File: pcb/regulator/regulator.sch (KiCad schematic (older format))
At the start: 16 parts, among them J1 Conn_01x04, J2 Conn_01x03, SW1 SW_Push, U1 STM32G071CBT6, Y1 32kHz, Y2 8MHz

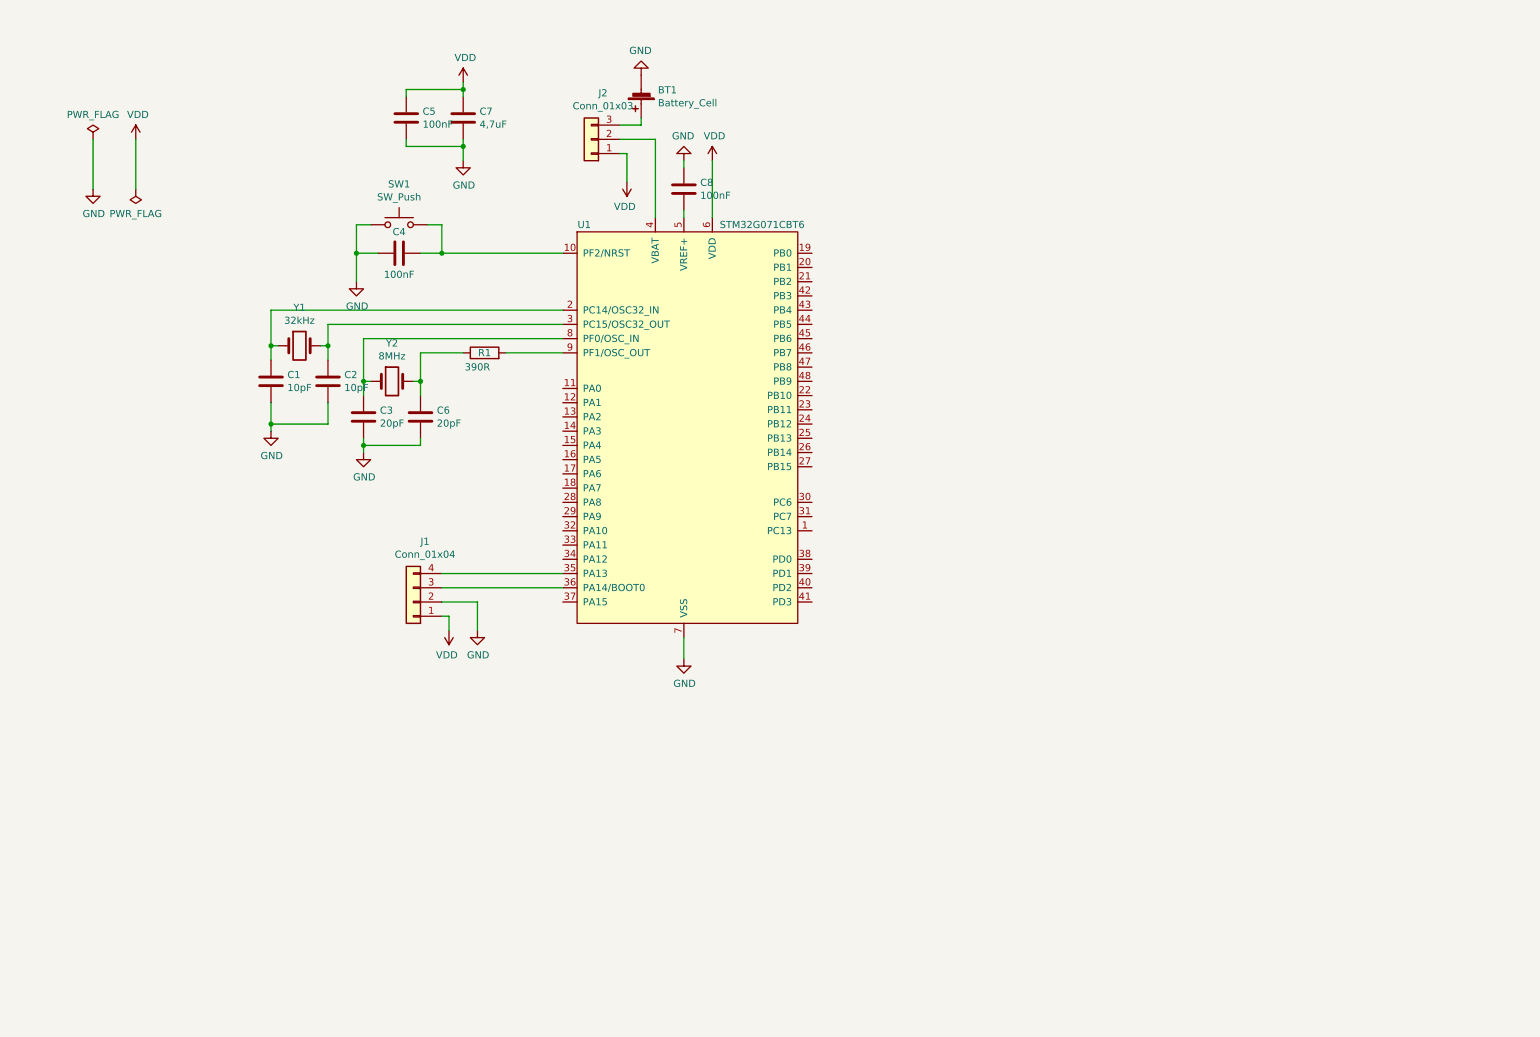
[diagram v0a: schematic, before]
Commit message: Device Schematic v1
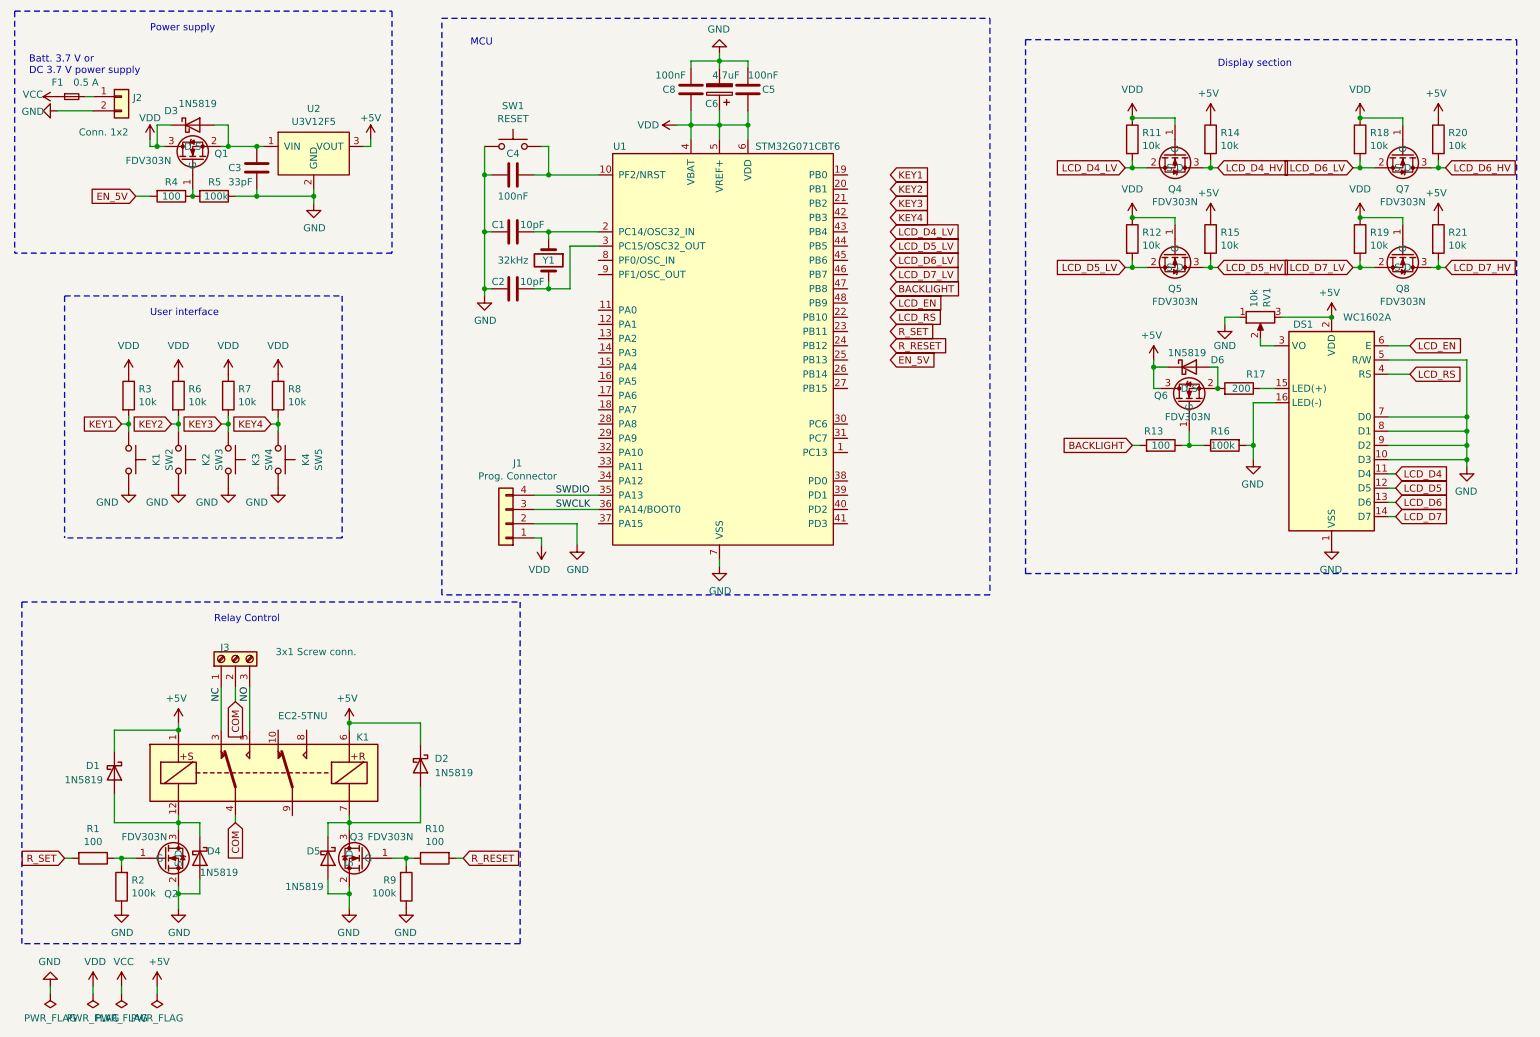
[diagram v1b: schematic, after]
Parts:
- removed BT1: Battery_Cell, symbol Device:Battery_Cell
- removed C6: 20pF, symbol Device:C
- removed C7: 4,7uF, symbol Device:C
- removed J2: Conn_01x03, symbol Connector_Generic:Conn_01x03
- removed Y2: 8MHz, symbol Device:Crystal
- added C6: 4.7uF, symbol Device:CP
- added D1, D2, D3, D4, D5, D6: 1N5819, Diode_THT:D_DO-41_SOD81_P10.16mm_Horizontal, symbol Diode:1N5819
- added DS1: WC1602A, Display:WC1602A, symbol Display_Character:WC1602A
- added F1: 0.5 A, symbol Device:Fuse_Small
- added J2: Conn. 1x2, symbol Connector_Generic:Conn_01x02
- added J3: 3x1 Screw conn., symbol Connector:Screw_Terminal_01x03
- added K1: EC2-5TNU, Relay_THT:Relay_DPDT_Kemet_EC2_DoubleCoil, symbol Relay:EC2-5TNU
- added Q1, Q2, Q3, Q4, Q5, Q6, Q7, Q8: FDV303N, Package_TO_SOT_SMD:SOT-23, symbol things:FDV303N
- added R10, R13, R4: 100, symbol Device:R
- added R11, R12, R14, R15, R18, R19, R20, R21, R3, R6, R7, R8: 10k, symbol Device:R
- added R16, R2, R5, R9: 100k, symbol Device:R
- added R17: 200, symbol Device:R
- added RV1: 10k, symbol Device:R_POT
- added SW2: K1, symbol Switch:SW_Push
- added SW3: K2, symbol Switch:SW_Push
- added SW4: K3, symbol Switch:SW_Push
- added SW5: K4, symbol Switch:SW_Push
- added U2: U3V12F5, Connector_PinHeader_2.54mm:PinHeader_1x03_P2.54mm_Vertical_SMD_Pin1Left, symbol things:U3V12F5
- C3: value 20pF -> 33pF
- J1: value Conn_01x04 -> Prog. Connector
- R1: value 390R -> 100
- SW1: value SW_Push -> RESET
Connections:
- net GND: now also C5.1, C6.2, D4.2 (A), D5.2 (A), DS1.1 (VSS), DS1.10 (D3), DS1.16 (LED(-)), DS1.5 (R/W), DS1.7 (D0), DS1.8 (D1), DS1.9 (D2), J2.2 (Pin_2), Q2.2 (S), Q3.2 (S), R16.2, R2.1, R5.1, R9.1, RV1.1, SW2.2, SW3.2, SW4.2, SW5.2, U2.2 (GND); no longer C5.2
- net VDD: now also C5.2, C8.2, U1.4 (VBAT), U1.5 (VREF+), C6.1, D3.1 (K), Q1.3 (D), Q4.1 (G), Q5.1 (G), Q7.1 (G), Q8.1 (G), R11.1, R12.1, R18.1, R19.1, R3.1, R6.1, R7.1, R8.1; no longer C5.1
- net SWDIO: now reaches J1.4 (Pin_4), U1.35 (PA13)
- net SWCLK: now reaches J1.3 (Pin_3), U1.36 (PA14/BOOT0)
- net at U1.8 (PF0/OSC_IN): no longer C3.1
- net at U1.9 (PF1/OSC_OUT): no longer R1.2
- net at R1.1: now also Q2.1 (G), R2.2
- new net: Q1.1 (G), R4.1, R5.2
- new net: C3.1, D3.2 (A), Q1.2 (S), U2.1 (VIN)
- new net: D1.2 (A), D4.1 (K), K1.12, Q2.3 (D)
- new net: Q3.1 (G), R10.1, R9.2
- new net: D2.2 (A), D5.1 (K), K1.7, Q3.3 (D)
- new net: Q6.1 (G), R13.1, R16.1
- new net: DS1.15 (LED(+)), R17.1
- new net: D6.2 (A), Q6.2 (S), R17.2
- new net: DS1.3 (VO), RV1.2
- new net: F1.2, J2.1 (Pin_1)
- new net +5V: D1.1 (K), D2.1 (K), D6.1 (K), DS1.2 (VDD), K1.1, K1.6, Q6.3 (D), R14.1, R15.1, R20.1, R21.1, RV1.3, U2.3 (VOUT)
- new net BACKLIGHT: R13.2
- new net COM: J3.2 (Pin_2), K1.4
- new net EN_5V: R4.2
- new net KEY1: R3.2, SW2.1
- new net KEY2: R6.2, SW3.1
- new net KEY3: R7.2, SW4.1
- new net KEY4: R8.2, SW5.1
- new net LCD_D4: DS1.11 (D4)
- new net LCD_D4_HV: Q4.3 (D), R14.2
- new net LCD_D4_LV: Q4.2 (S), R11.2
- new net LCD_D5: DS1.12 (D5)
- new net LCD_D5_HV: Q5.3 (D), R15.2
- new net LCD_D5_LV: Q5.2 (S), R12.2
- new net LCD_D6: DS1.13 (D6)
- new net LCD_D6_HV: Q7.3 (D), R20.2
- new net LCD_D6_LV: Q7.2 (S), R18.2
- new net LCD_D7: DS1.14 (D7)
- new net LCD_D7_HV: Q8.3 (D), R21.2
- new net LCD_D7_LV: Q8.2 (S), R19.2
- new net LCD_EN: DS1.6 (E)
- new net LCD_RS: DS1.4 (RS)
- new net NC: J3.1 (Pin_1), K1.3
- new net NO: J3.3 (Pin_3), K1.5
- new net R_RESET: R10.2
- new net R_SET: R1.2
- new net VCC: F1.1
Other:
- note added: "Batt. 3.7 V or\nDC 3.7 V power supply"
- note added: "Display section"
- note added: "MCU\n"
- note added: "Power supply"
- note added: "Relay Control"
- note added: "User interface"
- moved on the sheet: C1, C2, C4, C5, C8, J1, SW1, U1, Y1
